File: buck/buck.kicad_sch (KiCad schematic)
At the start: 2 parts, among them U1 LM2596S-12

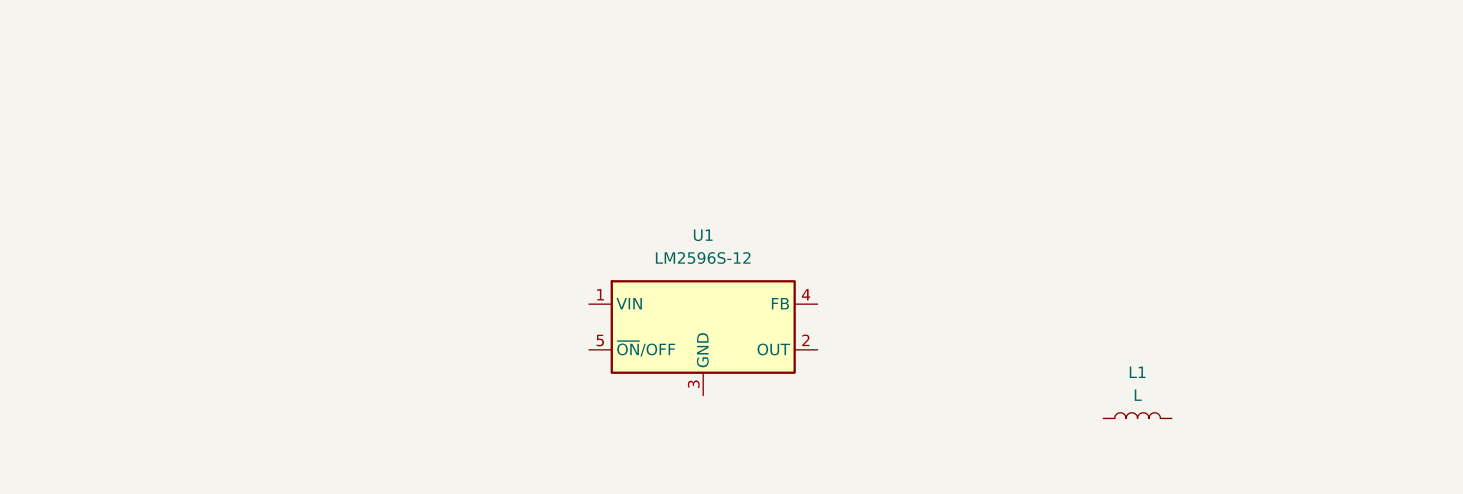
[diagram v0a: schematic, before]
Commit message: update
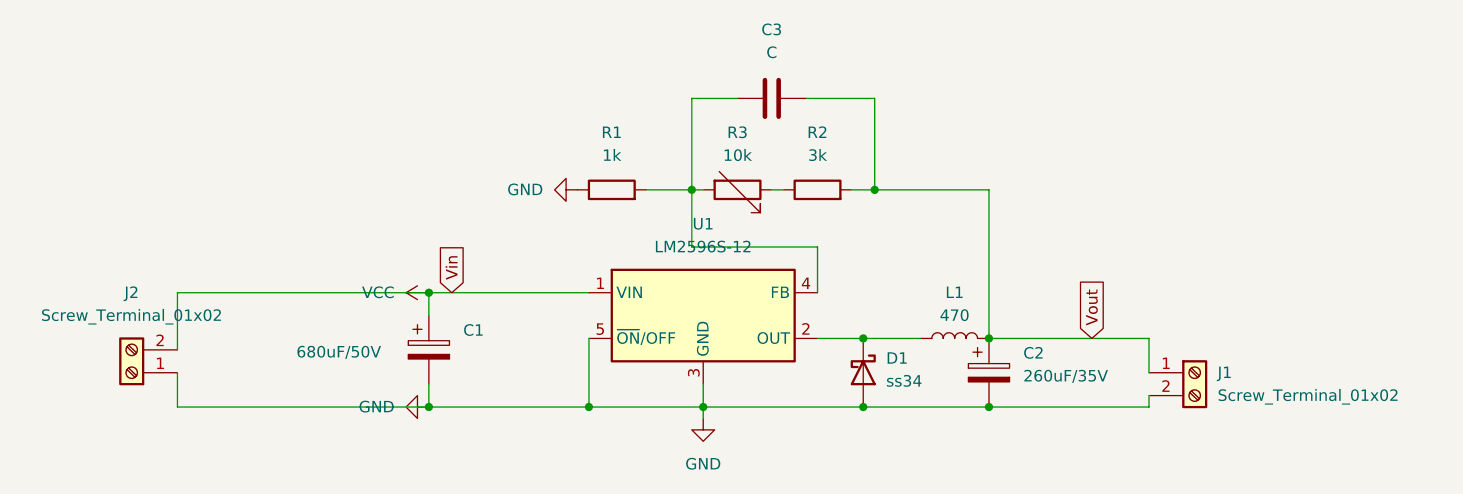
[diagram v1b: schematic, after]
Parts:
- added C1: 680uF/50V, symbol Device:C_Polarized
- added C2: 260uF/35V, symbol Device:C_Polarized
- added C3: C, symbol Device:C
- added D1: ss34, symbol Device:D_Schottky
- added J1, J2: Screw_Terminal_01x02, TerminalBlock_Phoenix:TerminalBlock_Phoenix_MKDS-1,5-2-5.08_1x02_P5.08mm_Horizontal, symbol Connector:Screw_Terminal_01x02
- added R1: 1k, symbol Device:R
- added R2: 3k, symbol Device:R
- added R3: 10k, symbol Device:R_Variable
- L1: value L -> 470
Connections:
- net VCC: now reaches U1.1 (VIN)
- net VCC: now also C1.1, J2.2 (Pin_2)
- net at U1.2 (OUT): now also L1.1, D1.1 (K)
- net GND: now reaches U1.3 (GND)
- net GND: now also U1.5 (~{ON}/OFF), C1.2, C2.2, D1.2 (A), J1.2 (Pin_2), J2.1 (Pin_1), R1.1
- net at U1.4 (FB): now also C3.1, R1.2, R3.2
- net Vout: now reaches L1.2
- net Vout: now also C2.1, C3.2, J1.1 (Pin_1), R2.2
- new net: R2.1, R3.1
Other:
- moved on the sheet: L1, U1
